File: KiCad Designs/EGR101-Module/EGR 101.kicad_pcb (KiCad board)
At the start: 2 copper layers, 42 x 27 mm, 20 parts, among them J1 GX12, J2 VEML7700-1, J3 VEML7700-2, J4 NEO-6M, U1 MAX3485, U2 LMR33630BDDA, U3 113991054

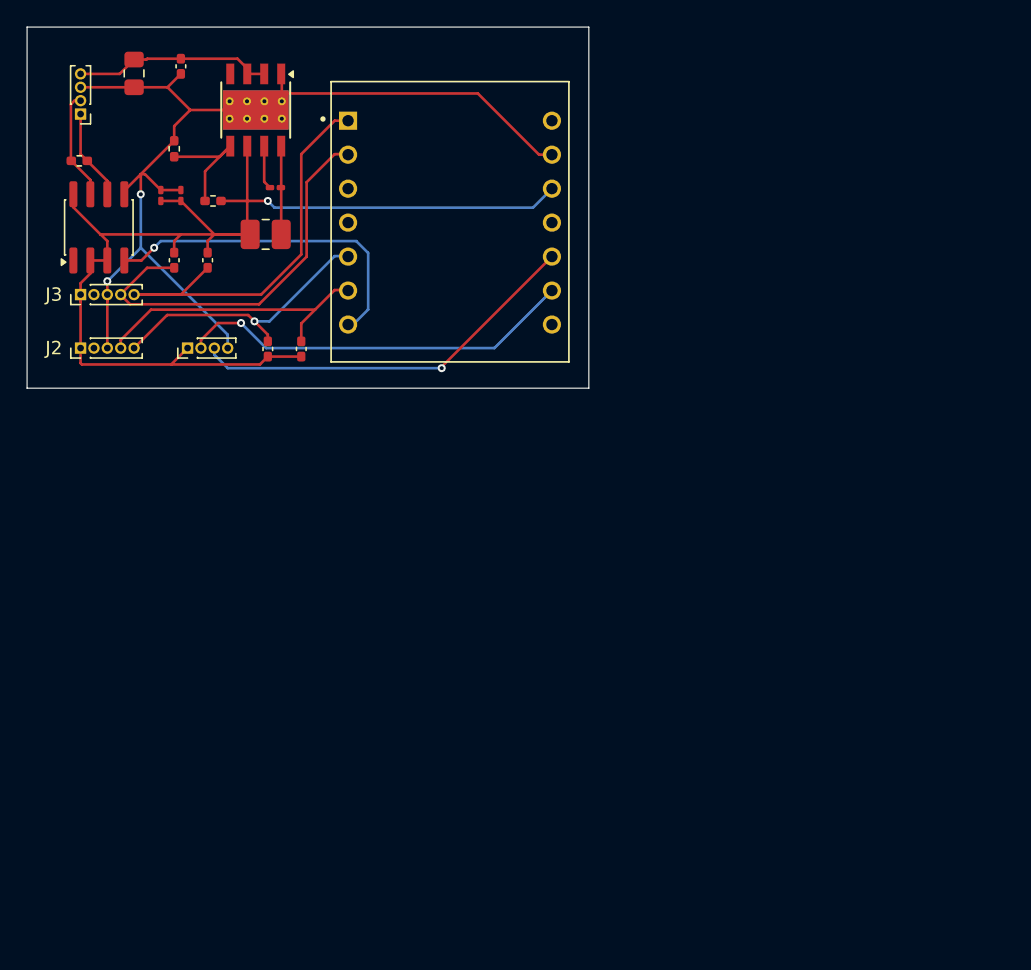
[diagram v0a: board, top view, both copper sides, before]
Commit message: More udaptes
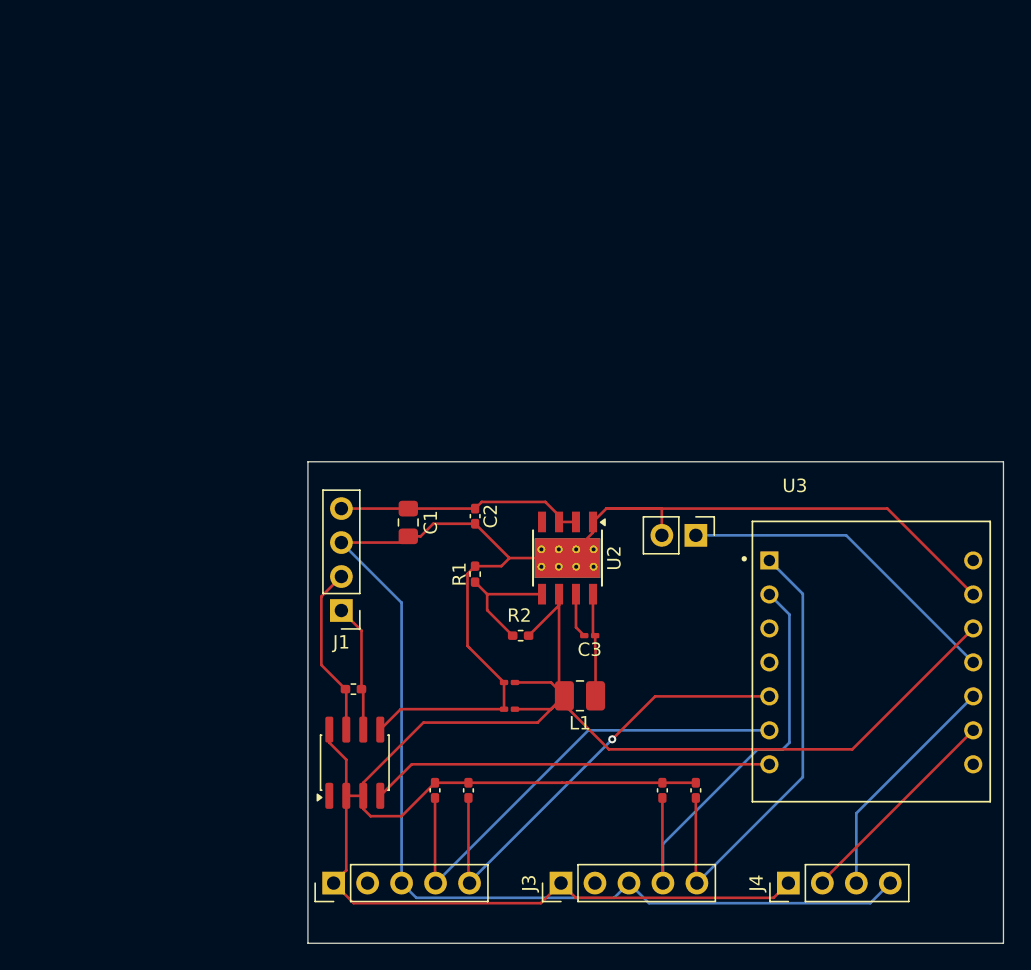
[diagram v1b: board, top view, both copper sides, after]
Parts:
- added J5: Switch, Connector_PinHeader_2.54mm:PinHeader_1x02_P2.54mm_Vertical, F.Cu at (115.0, 89.0)
- J1, J4: footprint Connector_PinHeader_1.00mm:PinHeader_1x04_P1.00mm_Vertical -> Connector_PinHeader_2.54mm:PinHeader_1x04_P2.54mm_Vertical
- J2, J3: footprint Connector_PinHeader_1.00mm:PinHeader_1x05_P1.00mm_Vertical -> Connector_PinHeader_2.54mm:PinHeader_1x05_P2.54mm_Vertical
- moved J4 60.1 mm to (121.9, 115.0)
- moved J3 56.8 mm to (104.9, 115.0)
- moved R4 53.9 mm to (112.5, 108.1)
- moved R8 53.9 mm to (115.0, 108.1)
- moved C4 46.4 mm to (101.1, 102.0), turned to 180 degrees
- moved U3 45.5 mm to (128.1, 98.4)
- moved R3 44.5 mm to (89.4, 100.5)
- moved U1 44.4 mm to (89.5, 106.0)
- moved J2 44.2 mm to (87.9, 115.0)
- moved C5 43.9 mm to (101.1, 100.0), turned to 180 degrees
- moved J1 41.9 mm to (88.5, 94.6)
- moved L1 41.7 mm to (106.3, 101.0)
- moved C3 40.9 mm to (107.1, 96.5)
- moved U2 40.8 mm to (105.4, 90.7)
- moved C2 40.2 mm to (98.5, 87.6)
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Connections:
- U3 pad 11: unconnected-(U3-D10-Pad11) -> Net-(J5-Pin_1)
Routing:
- net Net-(J1-Pin_3): track 78.4 -> 150.5 mm, vias 2 -> 0
- net Net-(J2-Pin_1): track 88.0 -> 152.2 mm, vias 1 -> 0
- net Net-(J5-Pin_1): track 0.00 -> 24.7 mm
- net Net-(J2-Pin_4): track 22.0 -> 36.2 mm
- net Net-(J4-Pin_2): track 29.9 -> 16.1 mm, vias 1 -> 0
- net Net-(J2-Pin_5): track 21.2 -> 34.9 mm
- net Net-(J4-Pin_3): track 29.8 -> 17.6 mm, vias 1 -> 0
- net Net-(U1-DI): track 25.4 -> 30.1 mm, vias 1 -> 0
- net Net-(J1-Pin_2): track 8.17 -> 12.8 mm
- net Net-(J1-Pin_4): track 14.9 -> 18.6 mm
- net Net-(J3-Pin_4): track 30.1 -> 33.8 mm
- net Net-(J3-Pin_5): track 32.1 -> 35.1 mm
- net Net-(J1-Pin_1): track 6.83 -> 9.58 mm
- net Net-(U2-SW): track 6.62 -> 7.68 mm
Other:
- board size 42 x 27 mm -> 52 x 36 mm
- board text removed: "4.7 kΩ"

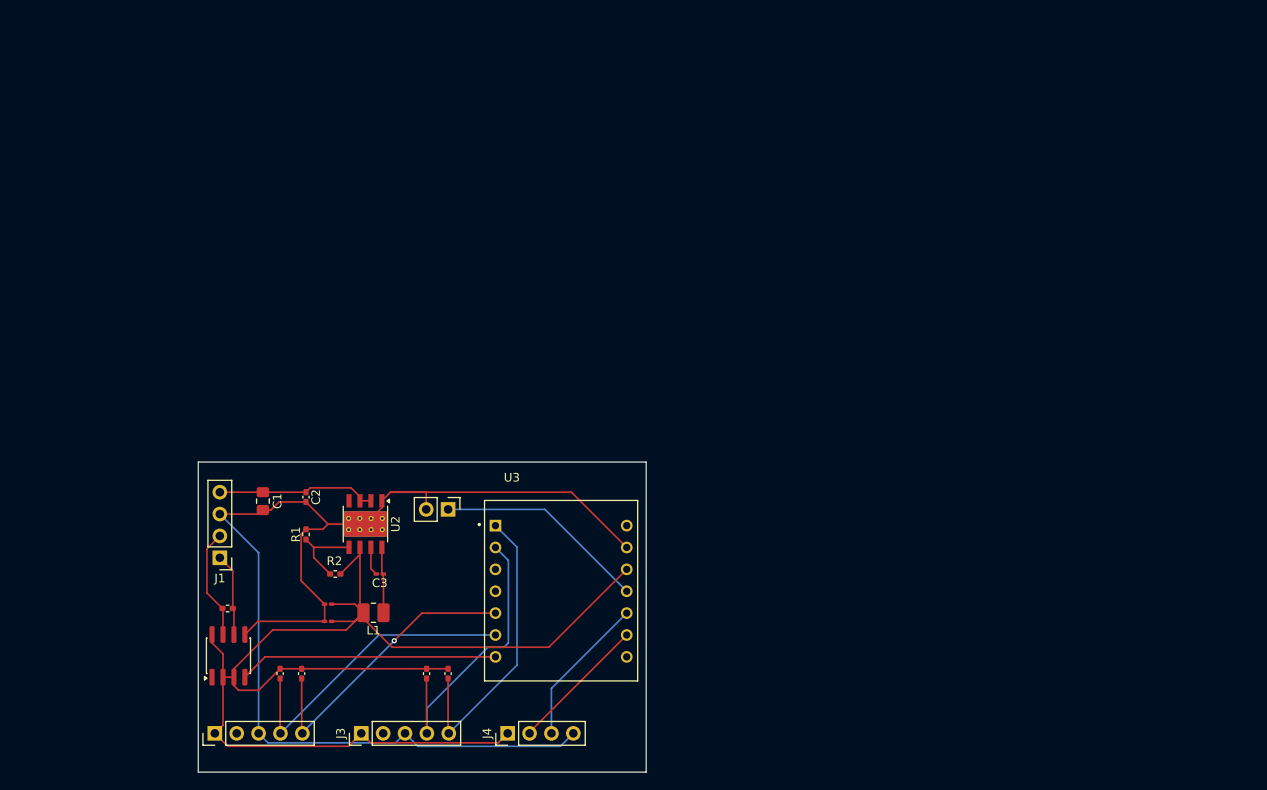
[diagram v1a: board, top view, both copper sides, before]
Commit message: Module V1.0 Done
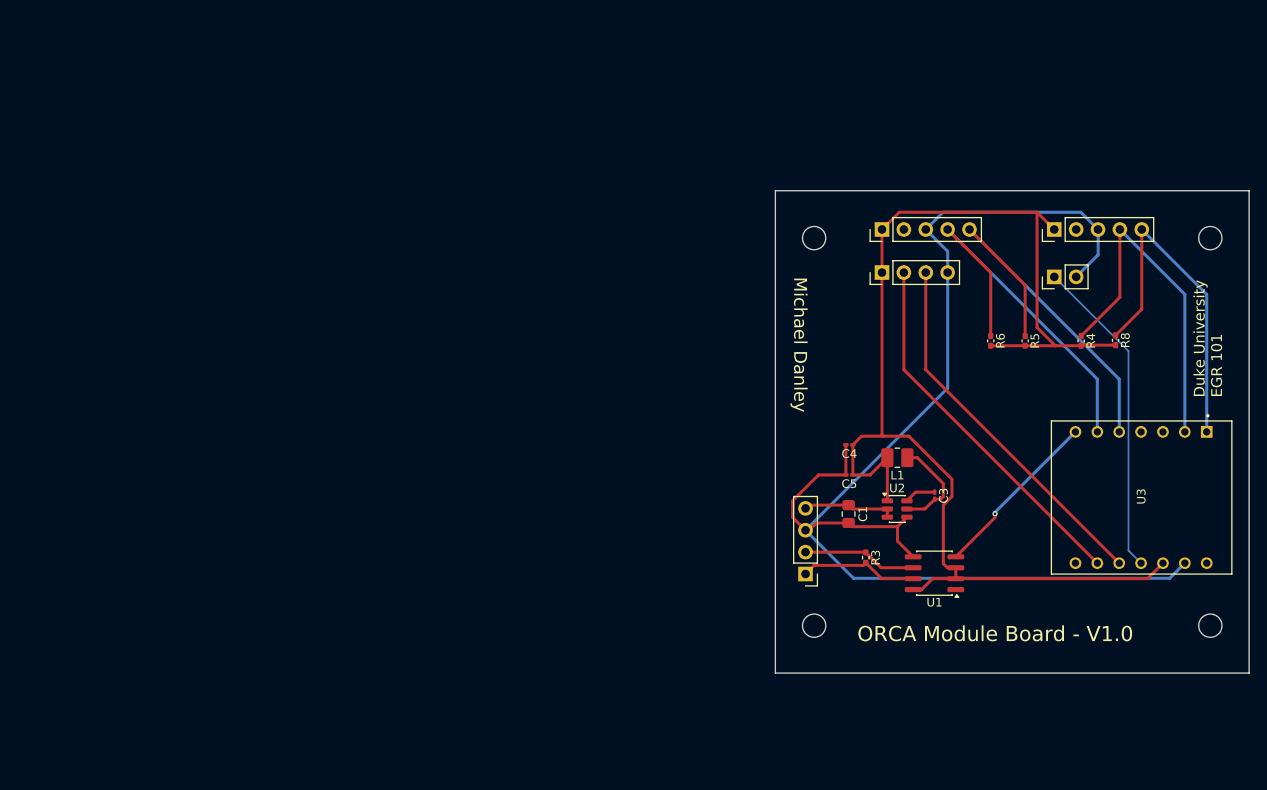
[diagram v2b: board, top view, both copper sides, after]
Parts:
- removed C2: 220 nF, Capacitor_SMD:C_0402_1005Metric_Pad0.74x0.62mm_HandSolder
- removed R1: 43.2 kΩ, Resistor_SMD:R_0402_1005Metric_Pad0.72x0.64mm_HandSolder
- removed R2: 100 kΩ, Resistor_SMD:R_0402_1005Metric_Pad0.72x0.64mm_HandSolder
- added H1: MountingHole, MountingHole:MountingHole_2.7mm, F.Cu at (203.5, 57.5)
- added H2: MountingHole, MountingHole:MountingHole_2.7mm, F.Cu at (203.5, 102.5)
- added H3: MountingHole, MountingHole:MountingHole_2.7mm, F.Cu at (157.5, 102.5)
- added H4: MountingHole, MountingHole:MountingHole_2.7mm, F.Cu at (157.5, 57.5)
- C3: value 0.1 uF -> 100 nF
- J1: value GX12 -> External Connection
- L1: value 2.2 uH -> 3.9 uH
- U2: value LMR33630BDDA -> AP63203WU; footprint Package_SO:Texas_HSOP-8-1EP_3.9x4.9mm_P1.27mm_ThermalVias -> Package_TO_SOT_SMD:TSOT-23-6
- moved J3 99.5 mm to (185.4, 56.5)
- moved J2 97.1 mm to (165.4, 56.5)
- moved R5 92.5 mm to (182.0, 69.4), turned to -90 degrees
- moved R6 91.1 mm to (178.0, 69.4), turned to -90 degrees
- moved R8 86.6 mm to (192.5, 69.4), turned to -90 degrees
- moved R4 85.3 mm to (188.5, 69.4), turned to -90 degrees
- moved U1 82.5 mm to (171.5, 96.4), turned to 180 degrees
- moved J5 75.4 mm to (185.4, 62.0), turned to 90 degrees
- moved R3 74.3 mm to (163.5, 94.6), turned to -90 degrees
- moved J4 68.9 mm to (165.4, 61.5)
- moved U3 68.3 mm to (195.5, 87.6), turned to -90 degrees
- moved J1 68.0 mm to (156.5, 96.5)
- moved C1 68.0 mm to (161.5, 89.5)
- moved C3 65.1 mm to (171.5, 87.4), turned to -90 degrees
- moved C4 63.9 mm to (161.6, 81.5)
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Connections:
- C3 pad 1: Net-(U2-SW) -> Net-(U2-BST)
- C3 pad 2: Net-(U2-BOOT) -> Net-(U2-SW)
- R3 pad 1: Net-(J1-Pin_1) -> Net-(J1-Pin_2)
- R3 pad 2: Net-(J1-Pin_2) -> Net-(J1-Pin_1)
- U1 pad 6: Net-(J1-Pin_1) -> Net-(J1-Pin_2)
- U1 pad 7: Net-(J1-Pin_2) -> Net-(J1-Pin_1)
- U2 pad 1: Net-(J1-Pin_3) -> Net-(J2-Pin_1)
- U2 pad 4: unconnected-(U2-PG-Pad4) -> Net-(J1-Pin_3)
- U2 pad 5: Net-(U2-FB) -> Net-(U2-SW)
- U2 pad 6: Net-(J2-Pin_1) -> Net-(U2-BST)
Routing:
- net Net-(J4-Pin_2): track 16.1 -> 43.0 mm
- net Net-(J4-Pin_3): track 17.6 -> 43.0 mm
- net Net-(J5-Pin_1): track 24.7 -> 37.4 mm
- net Net-(J2-Pin_5): track 34.9 -> 45.7 mm, vias 1 -> 0
- net Net-(U1-DI): track 30.1 -> 20.3 mm, vias 0 -> 1
- net Net-(U2-FB): track 9.26 -> 0.00 mm
- net Net-(J2-Pin_4): track 36.2 -> 45.1 mm
- net Net-(J1-Pin_4): track 18.6 -> 10.8 mm
- net Net-(J3-Pin_4): track 33.8 -> 40.9 mm
- net Net-(J3-Pin_5): track 35.1 -> 40.2 mm
- net Net-(J2-Pin_1): track 152.2 -> 147.4 mm
- net Net-(J1-Pin_1): track 9.58 -> 13.8 mm
- net Net-(U2-SW): track 7.68 -> 11.7 mm
- net Net-(U2-BST): track 0.00 -> 3.64 mm
- net Net-(U2-BOOT): track 3.36 -> 0.00 mm
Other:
- board size 52 x 36 mm -> 55 x 56 mm
- board text added: "Duke University EGR 101"
- board text added: "Michael Danley"
- board text added: "ORCA Module Board - V1.0"

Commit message: Chamber PCB Finished
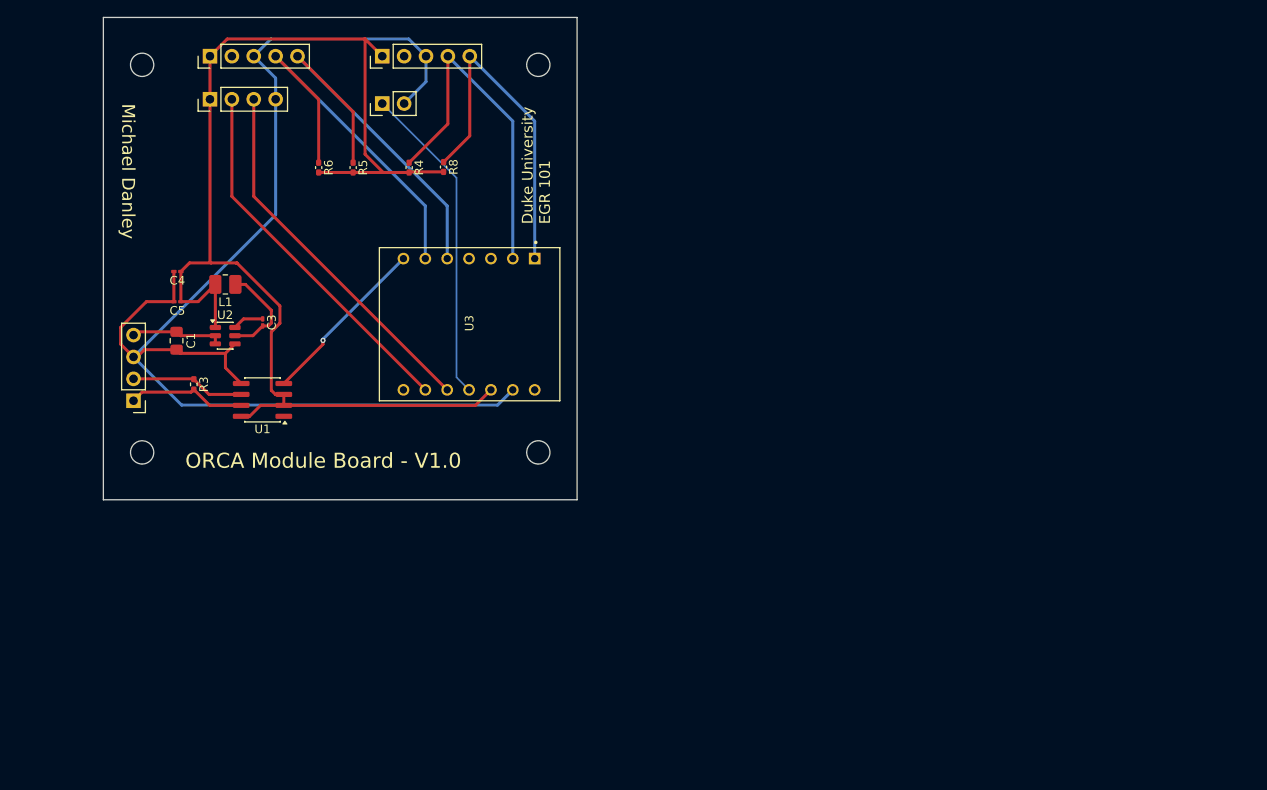
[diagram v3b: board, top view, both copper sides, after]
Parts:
- moved U3 80.6 mm to (117.5, 67.5)
- moved C1 80.6 mm to (83.5, 69.4)
- moved C3 80.6 mm to (93.5, 67.3)
- moved C4 80.6 mm to (83.6, 61.4)
- moved C5 80.6 mm to (83.6, 64.9)
- moved H1 80.6 mm to (125.5, 37.4)
- moved H2 80.6 mm to (125.5, 82.4)
- moved H3 80.6 mm to (79.5, 82.4)
- moved H4 80.6 mm to (79.5, 37.4)
- moved J1 80.6 mm to (78.5, 76.4)
- moved J2 80.6 mm to (87.4, 36.4)
- moved J3 80.6 mm to (107.4, 36.4)
- moved J4 80.6 mm to (87.4, 41.4)
- moved J5 80.6 mm to (107.4, 41.9)
- moved L1 80.6 mm to (89.1, 62.9)
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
